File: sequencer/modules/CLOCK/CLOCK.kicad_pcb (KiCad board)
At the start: 2 copper layers, 160 x 100 mm, 96 parts, among them J1 Card_Connector, J10 STRN, J11 STP, J12 XSTP, J13 REV, J2 CKOUT, J3 RST, J4 RIN, J5 CLR, J6 RND, J7 STUP, J8 STDN, J9 XCLK, Q1 2N3904, U1 40106, U2 40106, U3 4013, U4 40193, U6 40106, U7 TL082, U8 4514

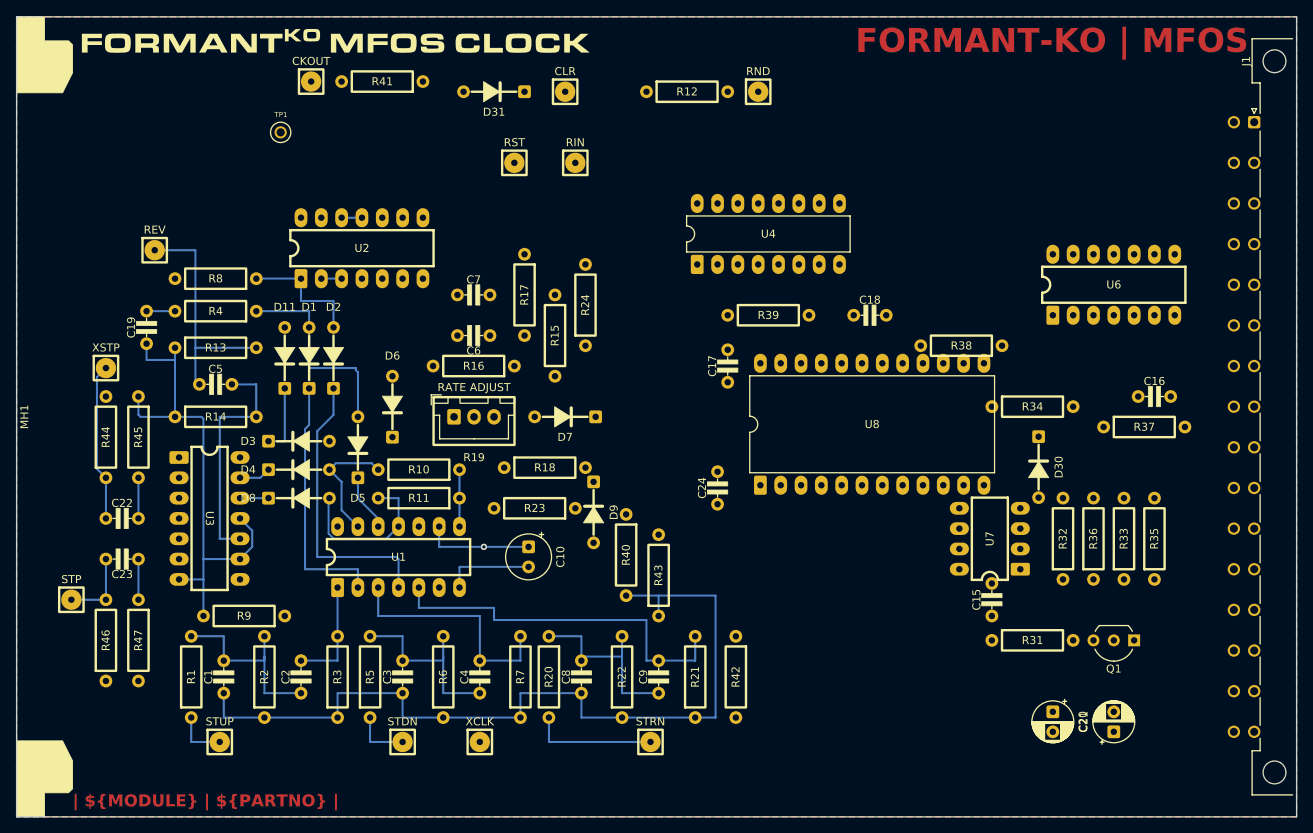
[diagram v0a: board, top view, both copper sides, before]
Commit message: sequencer clock pcb work
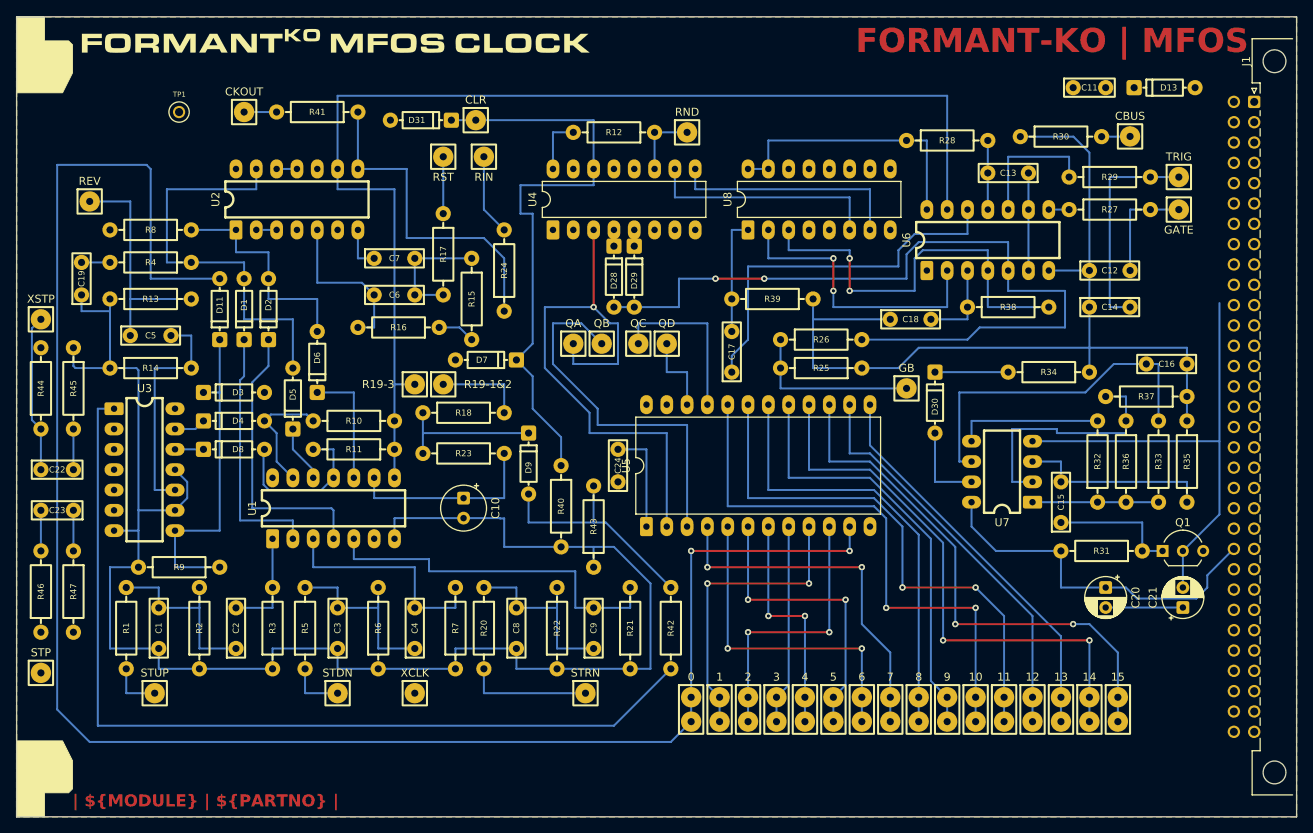
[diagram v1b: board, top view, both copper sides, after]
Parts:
- removed R19: 1M, FormantKO:PanelConnector_1x03
- added C11: 47p, FormantKO:C_Rect_160, F.Cu at (189.1, 53.9)
- added C12: 1n, FormantKO:C_Rect_200, F.Cu at (191.6, 76.7)
- added C13: 1n, FormantKO:C_Rect_200, F.Cu at (178.9, 64.5)
- added C14: 1n, FormantKO:C_Rect_200, F.Cu at (191.6, 81.3)
- added D13: DUS, FormantKO:DUS_300, F.Cu at (198.5, 53.9)
- added D28: DUS, FormantKO:DUS_300, F.Cu at (129.7, 77.5)
- added D29: DUS, FormantKO:DUS_300, F.Cu at (132.2, 77.5)
- added J14: R19-1&2, FormantKO:Wire_1x01_General, F.Cu at (108.3, 90.9)
- added J15: R19-3, FormantKO:Wire_1x01_General, F.Cu at (104.8, 90.9)
- added J16: QA, FormantKO:Wire_1x01_General, F.Cu at (124.6, 85.9)
- added J17: QB, FormantKO:Wire_1x01_General, F.Cu at (128.1, 85.9)
- added J18: QC, FormantKO:Wire_1x01_General, F.Cu at (132.7, 85.9)
- added J19: QD, FormantKO:Wire_1x01_General, F.Cu at (136.3, 85.9)
- added J20: 0, FormantKO:Wire_2x01_General, F.Cu at (139.3, 130.1)
- added J21: 1, FormantKO:Wire_2x01_General, F.Cu at (142.9, 130.1)
- added J22: 2, FormantKO:Wire_2x01_General, F.Cu at (146.4, 130.1)
- added J23: 3, FormantKO:Wire_2x01_General, F.Cu at (150.0, 130.1)
- added J24: 4, FormantKO:Wire_2x01_General, F.Cu at (153.5, 130.1)
- added J25: 5, FormantKO:Wire_2x01_General, F.Cu at (157.1, 130.1)
- added J26: 6, FormantKO:Wire_2x01_General, F.Cu at (160.7, 130.1)
- added J27: 7, FormantKO:Wire_2x01_General, F.Cu at (164.2, 130.1)
- added J28: 8, FormantKO:Wire_2x01_General, F.Cu at (167.8, 130.1)
- added J29: 9, FormantKO:Wire_2x01_General, F.Cu at (171.3, 130.1)
- added J30: 10, FormantKO:Wire_2x01_General, F.Cu at (174.9, 130.1)
- added J31: 11, FormantKO:Wire_2x01_General, F.Cu at (178.4, 130.1)
- added J32: 12, FormantKO:Wire_2x01_General, F.Cu at (182.0, 130.1)
- added J33: 13, FormantKO:Wire_2x01_General, F.Cu at (185.5, 130.1)
- added J34: 14, FormantKO:Wire_2x01_General, F.Cu at (189.1, 130.1)
- added J35: 15, FormantKO:Wire_2x01_General, F.Cu at (192.7, 130.1)
- added J36: GB, FormantKO:Wire_1x01_General, F.Cu at (166.2, 91.4)
- added J37: CBUS, FormantKO:Wire_1x01_General, F.Cu at (194.2, 59.9)
- added J38: TRIG, FormantKO:Wire_1x01_General, F.Cu at (200.3, 65.0)
- added J39: GATE, FormantKO:Wire_1x01_General, F.Cu at (200.3, 69.1)
- added R25: 4K7, FormantKO:R_Axial_Horizontal_400, F.Cu at (155.6, 88.9)
- added R26: 100k, FormantKO:R_Axial_Horizontal_400, F.Cu at (155.6, 85.3)
- added R27: 1k, FormantKO:R_Axial_Horizontal_400, F.Cu at (191.6, 69.1)
- added R28: 100k, FormantKO:R_Axial_Horizontal_400, F.Cu at (171.3, 60.5)
- added R29: 1k, FormantKO:R_Axial_Horizontal_400, F.Cu at (191.6, 65.0)
- added R30: 3k, FormantKO:R_Axial_Horizontal_400, F.Cu at (185.5, 60.0)
- added U8: HEF4094B, FormantKO:DIP-16, F.Cu at (155.3, 67.8)
- C1, C15, C16, C17, C18, C2, C3, C4, C5, C6, C7, C8, C9: footprint FormantKO:C_Rect_160 -> FormantKO:C_Rect_200
- J1: value Card_Connector -> Sequencer Bus Connector; footprint FormantKO:Card_Connector -> FormantKO:BusConnector_Full_Male_Horizontal
- MH1: footprint FormantKO:Card_Bracket -> FormantKO:CardBracket
- moved U4 18.5 mm to (130.9, 67.8)
- moved C21 17.8 mm to (200.8, 118.8)
- moved C20 16.9 mm to (191.1, 116.3)
- moved U6 16.7 mm to (176.4, 72.9)
- moved D30 15.3 mm to (169.8, 93.2)
- moved U5 15.2 mm to (147.7, 101.1)
- moved C15 14.9 mm to (185.5, 105.7)
- moved R31 14.1 mm to (190.6, 111.8), turned to 180 degrees
- moved TP1 13.0 mm to (75.3, 56.9)
- moved C24 12.8 mm to (130.2, 101.1)
- moved R18 12.3 mm to (110.9, 94.5)
- moved D7 12.2 mm to (113.7, 87.9)
- moved Q1 11.7 mm to (198.2, 111.8), turned to 0 degrees
- moved J5 11.7 mm to (112.4, 57.9)
- moved J4 11.5 mm to (113.4, 62.5)
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- renumbered U8 to U5
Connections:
- D7 pad 2: RST -> Net-(D7-A)
- J1 pad a18: unconnected-(J1-+5V-Pada18) -> +5V
- J1 pad b18: unconnected-(J1-+5V-Padb18) -> +5V
- R17 pad 1: Net-(R17-Pad1) -> RST
- R18 pad 2: Net-(R18-Pad2) -> R19-1&2
- TP1 pad 1: RST -> Net-(D7-A)
- U2 pad 6: RST -> Net-(D7-A)
- U5 pad 10: unconnected-(U8-Q2-Pad10) -> S-2
- U5 pad 11: unconnected-(U8-Q0-Pad11) -> FWD
- U5 pad 13: unconnected-(U8-Q13-Pad13) -> S-13
- U5 pad 14: unconnected-(U8-Q12-Pad14) -> S-12
- U5 pad 15: unconnected-(U8-Q15-Pad15) -> S-15
- U5 pad 16: unconnected-(U8-Q14-Pad16) -> S-14
- U5 pad 17: unconnected-(U8-Q9-Pad17) -> S-9
- U5 pad 18: unconnected-(U8-Q8-Pad18) -> S-8
- U5 pad 19: unconnected-(U8-Q11-Pad19) -> S-11
- U5 pad 20: unconnected-(U8-Q10-Pad20) -> S-10
- U5 pad 4: unconnected-(U8-Q7-Pad4) -> S-7
- U5 pad 5: unconnected-(U8-Q6-Pad5) -> S-6
- U5 pad 6: unconnected-(U8-Q5-Pad6) -> S-5
- U5 pad 7: unconnected-(U8-Q4-Pad7) -> S-4
- U5 pad 8: unconnected-(U8-Q3-Pad8) -> S-3
- U5 pad 9: unconnected-(U8-Q1-Pad9) -> S-1
- U6 pad 10: unconnected-(U6-Pad10) -> Net-(R29-Pad1)
- U6 pad 11: unconnected-(U6-Pad11) -> Net-(C13-Pad2)
- U6 pad 5: unconnected-(U6-Pad5) -> Net-(D28-A)
- U6 pad 6: unconnected-(U6-Pad6) -> Net-(C13-Pad1)
- U6 pad 8: unconnected-(U6-Pad8) -> Net-(R27-Pad1)
- U6 pad 9: unconnected-(U6-Pad9) -> Net-(C13-Pad1)
- U7 pad 4: GND -> -15V
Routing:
- net FWD: track 0.00 -> 228.5 mm, vias 0 -> 2
- net GND: track 180.3 -> 342.6 mm
- net CLK: track 7.11 -> 147.8 mm
- net Net-(U3A-Q): track 0.00 -> 116.2 mm
- net +15V: track 3.56 -> 108.8 mm
- net Net-(D28-A): track 0.00 -> 100.3 mm, vias 0 -> 2
- net CLR: track 0.00 -> 74.8 mm
- net QA: track 0.00 -> 72.2 mm, vias 0 -> 1
- net S-10: track 0.00 -> 69.7 mm, vias 0 -> 2
- net S-14: track 0.00 -> 69.3 mm, vias 0 -> 2
- net S-11: track 0.00 -> 67.5 mm, vias 0 -> 2
- net S-15: track 0.00 -> 67.4 mm, vias 0 -> 2
- net -15V: track 0.00 -> 60.8 mm
- net S-8: track 0.00 -> 55.1 mm
- net S-9: track 0.00 -> 53.8 mm
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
